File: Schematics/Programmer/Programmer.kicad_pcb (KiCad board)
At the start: 2 copper layers, 55.5 x 27.7 mm, 17 parts, among them J1 USB_C_Receptacle_USB2.0, J2 SubModule, J3 I2C example, SW1 SEL_SEL, SW2 RESET, U1 AP2112K-3.3

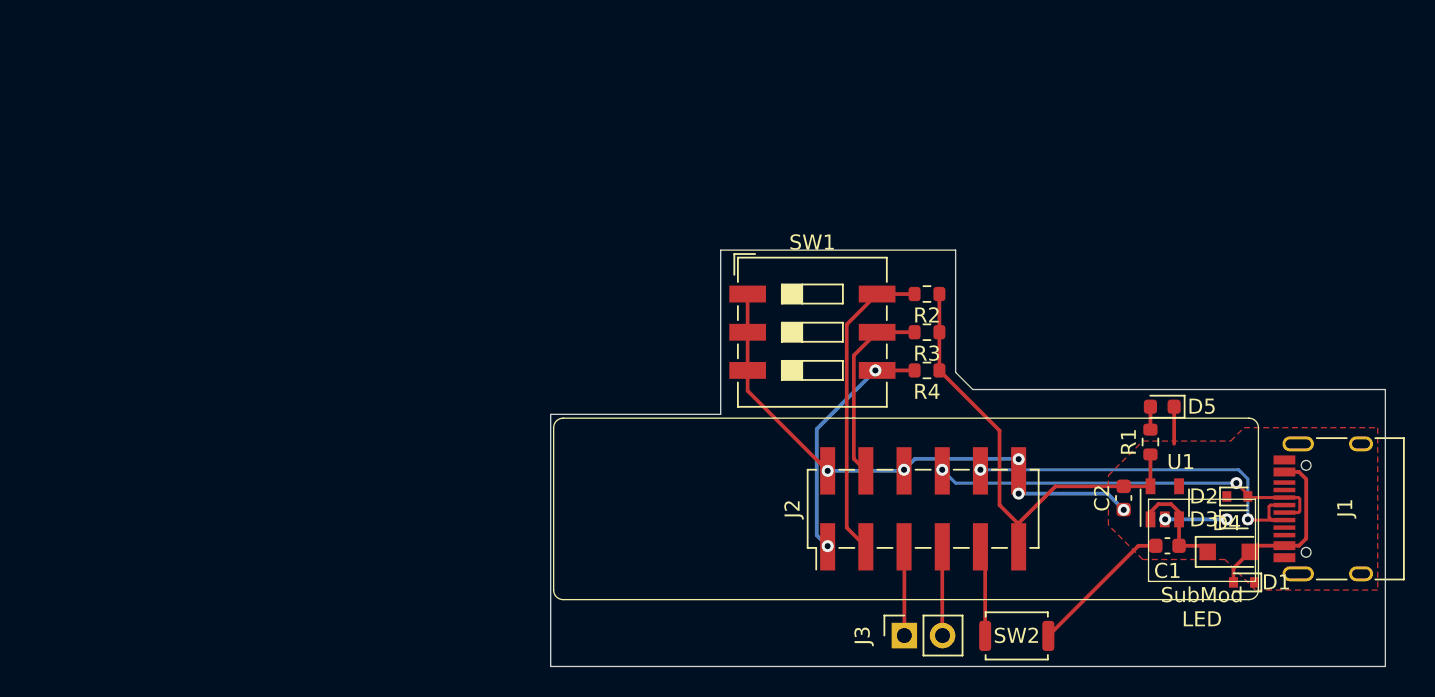
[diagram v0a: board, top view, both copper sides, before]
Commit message: Programmer completed
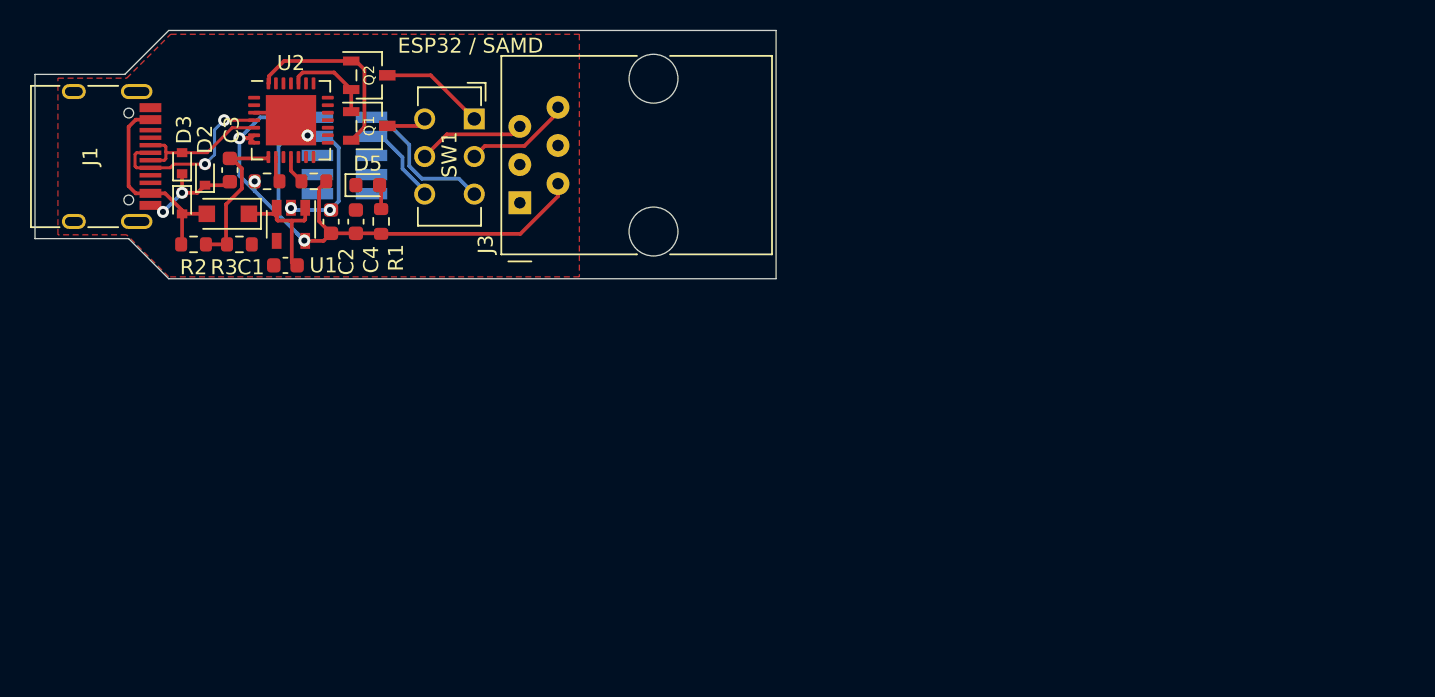
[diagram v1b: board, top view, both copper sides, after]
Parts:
- removed SW2: RESET, Button_Switch_SMD:SW_Push_SPST_NO_Alps_SKRK
- added C3: 10uF, Capacitor_SMD:C_0603_1608Metric, F.Cu at (105.4, 73.4)
- added C4: 10uF, Capacitor_SMD:C_0603_1608Metric, F.Cu at (113.8, 76.8)
- added Q1: DTC114T, libs:SOT346, F.Cu at (114.7, 70.5)
- added Q2: DTC114T, libs:SOT346, F.Cu at (114.7, 67.1)
- added R5: 10K, Resistor_SMD:R_0603_1608Metric, F.Cu at (111.0, 74.2)
- added U2: CP2102N-A01-GQFN28, Package_DFN_QFN:QFN-28-1EP_5x5mm_P0.5mm_EP3.35x3.35mm, F.Cu at (109.5, 70.1)
- D1, D2, D3: value LESD5D5.0CT1G -> LESD5
- D4: value 1N5819HW-7-F -> 1N5819HW
- J1: value USB_C_Receptacle_USB2.0 -> USB_C
- J2: value SubModule -> J-link; footprint Connector_PinHeader_2.54mm:PinHeader_2x06_P2.54mm_Vertical_SMD -> Connector_PinSocket_1.27mm:PinSocket_2x05_P1.27mm_Vertical_SMD; moved to B.Cu
- J3: value I2C example -> RJ12; footprint Connector_PinSocket_2.54mm:PinSocket_1x02_P2.54mm_Vertical -> Connector_RJ:RJ12_Amphenol_54601
- R2: value PullUp -> 22.1K
- R3: value PullUp -> 47.5K
- R4: value PullUp -> 1K
- SW1: value SEL_SEL -> ESP/SAMD; footprint Button_Switch_SMD:SW_DIP_SPSTx03_Slide_9.78x9.8mm_W8.61mm_P2.54mm -> Button_Switch_THT:SW_CuK_JS202011CQN_DPDT_Straight
- moved J1 86.7 mm to (96.1, 72.5), turned to -90 degrees
- moved D1 75.0 mm to (102.2, 75.6), turned to -90 degrees
- moved D3 74.1 mm to (102.2, 73.0), turned to 90 degrees
- moved D2 71.9 mm to (103.8, 73.7), turned to 90 degrees
- moved D4 70.2 mm to (105.3, 76.3), turned to 180 degrees
- moved C1 61.5 mm to (109.1, 79.8)
- moved U1 61.0 mm to (109.5, 77.0), turned to -90 degrees
- moved C2 55.8 mm to (112.1, 76.8), turned to -90 degrees
- moved D5 54.8 mm to (114.6, 74.4), turned to 0 degrees
- moved R1 53.2 mm to (115.5, 76.8)
- moved R2 48.9 mm to (103.0, 78.4), turned to 0 degrees
- moved R3 46.1 mm to (106.0, 78.4)
- moved R4 45.6 mm to (107.9, 74.2), turned to 0 degrees
- moved J2 45.1 mm to (113.0, 72.4), turned to 180 degrees
- moved J3 38.5 mm to (124.7, 75.6)
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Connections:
- J2 pad 1: /SEL3 -> +3V3
- J2 pad 10: /D- -> (no net)
- J2 pad 2: GND -> /SWD
- J2 pad 3: /SEL1 -> GND
- J2 pad 4: /SEL2 -> /SWC
- J2 pad 5: /SM_I2C_SDA -> (no net)
- J2 pad 6: GND -> (no net)
- J2 pad 7: /SM_I2C_SCL -> (no net)
- J2 pad 8: /D+ -> (no net)
- J2 pad 9: /RESET -> (no net)
- J3 pad 1: /SM_I2C_SDA -> /TX
- J3 pad 2: /SM_I2C_SCL -> +3V3
- R2 pad 1: +3V3 -> VBUS
- R2 pad 2: /SEL1 -> Net-(C3-Pad1)
- R3 pad 1: +3V3 -> GND
- R3 pad 2: /SEL2 -> Net-(C3-Pad1)
- R4 pad 2: /SEL3 -> Net-(R4-Pad2)
- SW1 pad 1: GND -> /EN
- SW1 pad 2: GND -> /D0
- SW1 pad 3: GND -> /SWD
- SW1 pad 4: /SEL3 -> /IO0
- SW1 pad 5: /SEL2 -> /D1
- SW1 pad 6: /SEL1 -> /SWC
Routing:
- net GND: track 53.0 -> 21.4 mm, vias 7 -> 5
- net /SEL1: track 20.7 -> 0.00 mm
- net /D-: track 26.2 -> 9.53 mm, vias 2 -> 0
- net +3V3: track 32.5 -> 48.9 mm, vias 0 -> 3
- net /SEL3: track 16.2 -> 0.00 mm, vias 2 -> 0
- net /D+: track 26.6 -> 12.4 mm
- net /SEL2: track 12.7 -> 0.00 mm
- net /~DTR: track 0.00 -> 12.6 mm
- net Net-(C3-Pad1): track 0.00 -> 10.7 mm
- net /SWD: track 0.00 -> 9.77 mm
- net /D1: track 0.00 -> 7.16 mm
- net /D0: track 0.00 -> 7.12 mm
- net /EN: track 0.00 -> 6.99 mm
- net /RESET: track 6.05 -> 0.00 mm
- net /~RTS: track 0.00 -> 6.01 mm
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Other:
- board size 55.5 x 27.7 mm -> 49.3 x 16.5 mm
- board text added: "ESP32 / SAMD"
- board text removed: "SubMod LED"
